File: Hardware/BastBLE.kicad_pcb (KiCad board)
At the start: 2 copper layers, 50.8 x 22.9 mm, 39 parts, among them J1 Conn_Battery, J2 SWD, J3 Conn_left, J4 Conn_right, P1 USB_C_Plug_USB2.0, Q1 DMG3415U-7, SW1 RESET, U1 AP2112K-3.3, U2 E73-2G4M08S1C, U3 MCP73831-2-OT, U4 W25Q32JVSS, Y1 32Khz

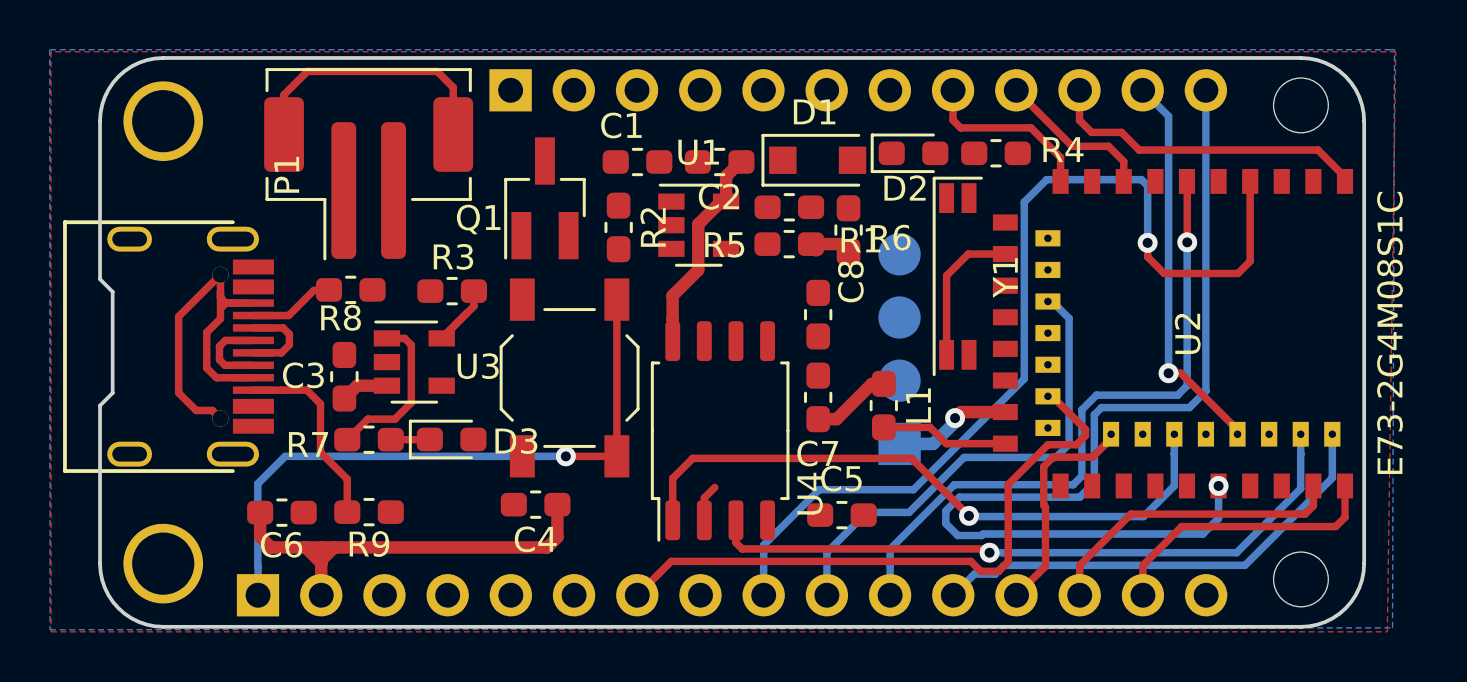
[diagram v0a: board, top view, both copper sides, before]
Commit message: routeo D
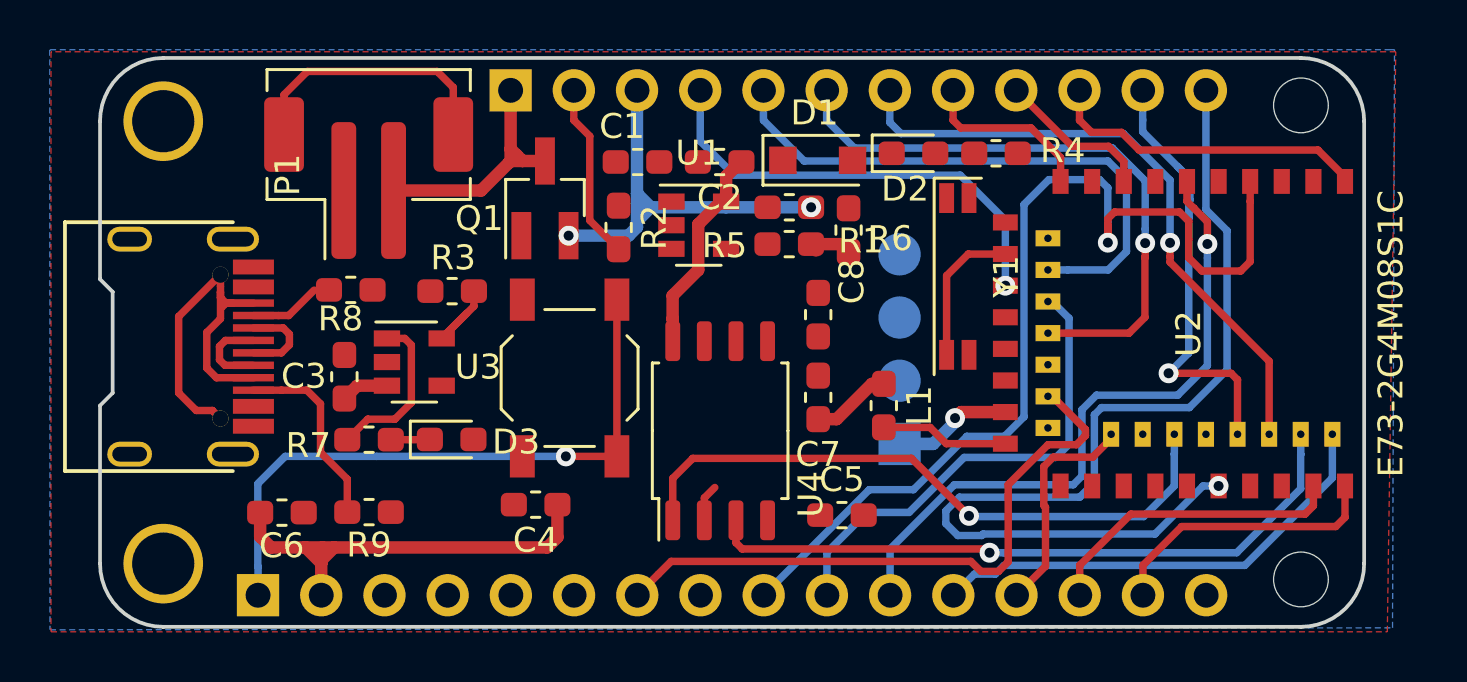
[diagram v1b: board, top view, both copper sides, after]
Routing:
- net /D10: track 0.00 -> 25.4 mm, vias 0 -> 1
- net /D11: track 0.00 -> 24.7 mm, vias 0 -> 1
- net /D12: track 0.00 -> 23.1 mm
- net /D13: track 0.00 -> 18.2 mm, vias 0 -> 1
- net VBUS: track 0.00 -> 17.0 mm, vias 0 -> 2
- net +BATT: track 1.92 -> 12.4 mm
- net /EN: track 0.00 -> 7.13 mm
- net /SCL: track 15.7 -> 19.8 mm
- net /A4: track 38.5 -> 40.8 mm
- net /SCK: track 26.3 -> 27.0 mm
